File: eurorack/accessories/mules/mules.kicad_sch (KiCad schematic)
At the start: 5 parts, among them J1 AudioPlug2, J2 AudioPlug2, J3 AudioJack3

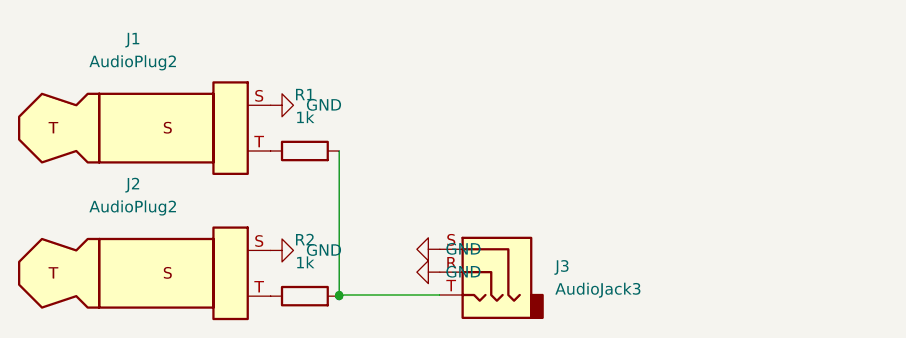
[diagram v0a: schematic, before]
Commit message: final mules v1 design
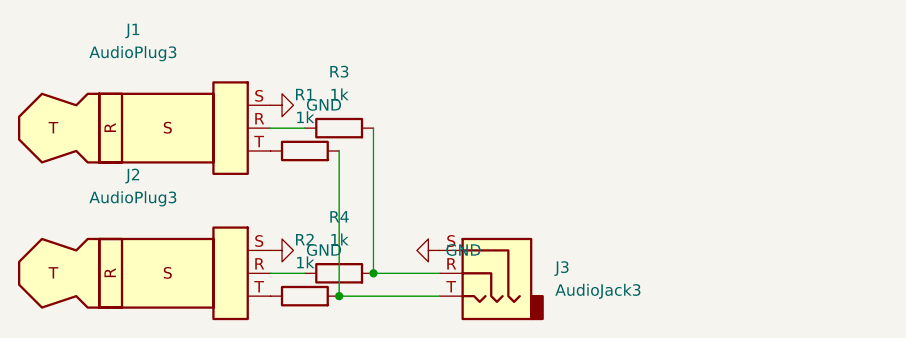
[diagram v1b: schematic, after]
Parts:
- removed J1, J2: AudioPlug2, Pale Slim Ghost:Kobiconn 173-35MPTIP-EX 3.5mm Audio Plug, symbol Connector:AudioPlug2
- added J1, J2: AudioPlug3, Pale Slim Ghost:Plug_3.5mm_CUI_SP-3533, symbol Connector:AudioPlug3
- added R3, R4: 1k, Resistor_SMD:R_0805_2012Metric_Pad1.20x1.40mm_HandSolder, symbol Device:R
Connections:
- net GND: now also J1.S, J2.S; no longer J3.R
- net at R2.1: now also J2.T
- net at R1.1: now also J1.T
- new net: J2.R, R4.1
- new net: J3.R, R3.2, R4.2
- new net: J1.R, R3.1

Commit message: assorted changes ig from opening things in kicad 7
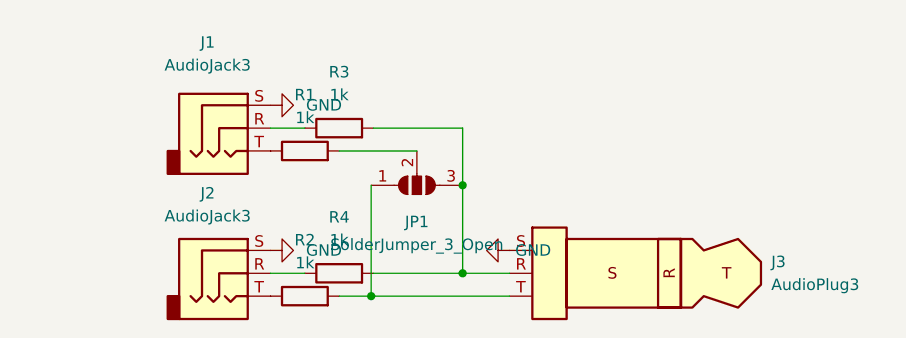
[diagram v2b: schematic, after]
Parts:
- removed J2: AudioPlug3, Pale Slim Ghost:Plug_3.5mm_CUI_SP-3533, symbol Connector:AudioPlug3
- added J2: AudioJack3, Connector_Audio:Jack_3.5mm_CUI_SJ-3523-SMT_Horizontal, symbol Connector:AudioJack3
- added JP1: SolderJumper_3_Open, Jumper:SolderJumper-3_P1.3mm_Open_RoundedPad1.0x1.5mm, symbol Jumper:SolderJumper_3_Open
- renumbered J3 to J1, J1 to J3
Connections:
- net GND: now also J2.S
- net at R4.1: now also J2.R
- net at R2.1: now also J2.T
- net at R3.2, R4.2: now also J3.R, JP1.3 (B); no longer J1.R
- net at R3.1: now also J1.R; no longer J3.R
- net at J3.T: now also R2.2, JP1.1 (A); no longer R1.1
- new net: JP1.2 (C), R1.2
- new net: J1.T, R1.1
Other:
- moved on the sheet: J1, J3
